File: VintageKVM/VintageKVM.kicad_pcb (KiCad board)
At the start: 2 copper layers, 164 parts, among them J1 Micro USB, J10 DE15_Receptacle_HighDensity_M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, J12 DE15_Receptacle_HighDensity_M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, J14 DE15_Receptacle_HighDensity_M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, J16 DE15_Receptacle_HighDensity_M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, J4 Conn_02x10_Odd_Even, J5 Conn_01x20_Pin, J6 Conn_01x20_Pin, J8 DE15_Receptacle_HighDensity_M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, Q1 BSS138, Q10 BSS138, Q2 BSS138, Q3 BSS138, Q4 BSS138, Q5 BSS138, Q6 BSS138, Q7 BSS138, Q8 BSS138, Q9 BSS138, U2 TS5V522CPWR, U3 TS5V522CPWR

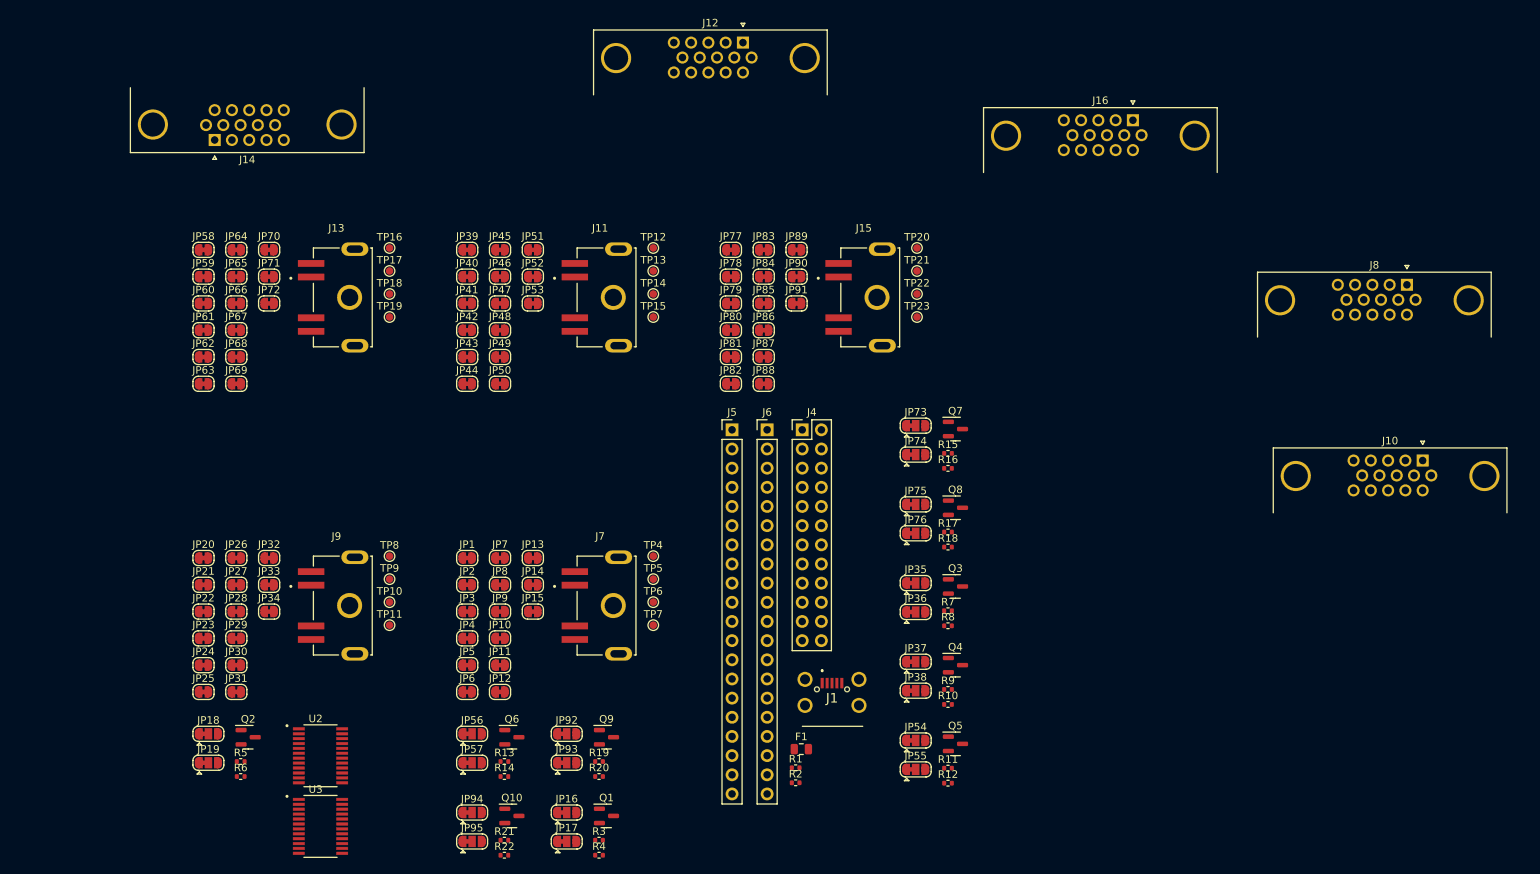
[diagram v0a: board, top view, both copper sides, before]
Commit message: started layout
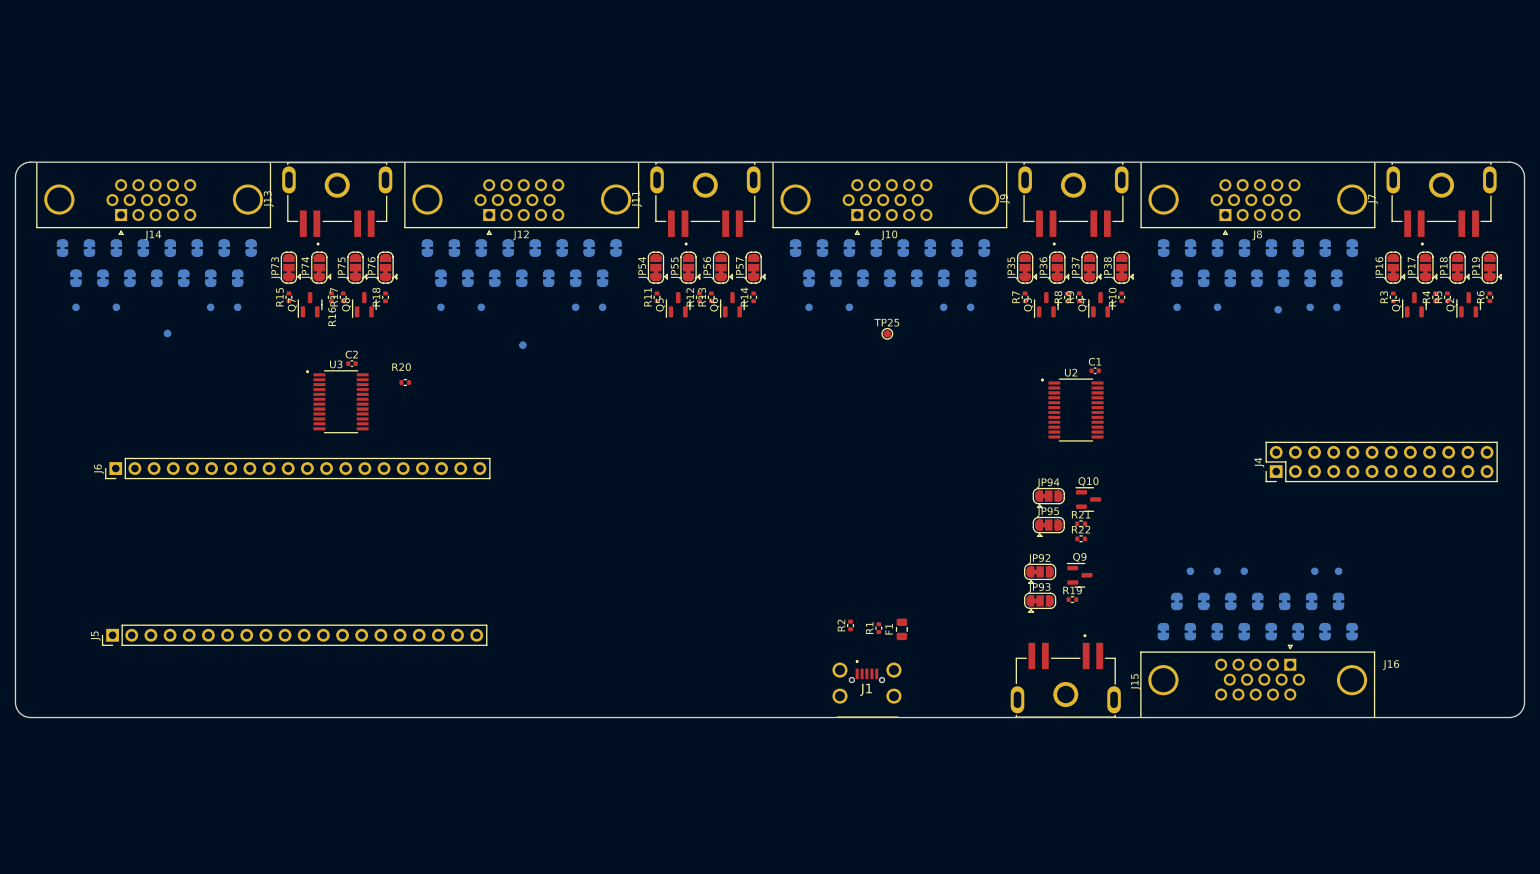
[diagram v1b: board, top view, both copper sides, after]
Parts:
- added C1: 100nF, Capacitor_SMD:C_0402_1005Metric, F.Cu at (183.1, 67.7)
- added C2: 100nF, Capacitor_SMD:C_0402_1005Metric, F.Cu at (84.6, 66.7)
- added TP24: TestPoint_Small, TestPoint:TestPoint_Pad_D1.0mm, B.Cu at (207.3, 59.5)
- added TP25: TestPoint_Small, TestPoint:TestPoint_Pad_D1.0mm, F.Cu at (155.6, 62.8)
- added TP26: TestPoint_Small, TestPoint:TestPoint_Pad_D1.0mm, B.Cu at (107.2, 64.2)
- added TP27: TestPoint_Small, TestPoint:TestPoint_Pad_D1.0mm, B.Cu at (60.1, 62.7)
- added TP28: TestPoint_Small, TestPoint:TestPoint_Pad_D1.0mm, B.Cu at (202.9, 94.2)
- JP1, JP10, JP11, JP12, JP13, JP14, JP15, JP2, JP20, JP21, JP22, JP23, JP24, JP25, JP26, JP27, JP28, JP29, JP3, JP30, JP31, JP32, JP33, JP34, JP39, JP4, JP40, JP41, JP42, JP43, JP44, JP45, JP46, JP47, JP48, JP49, JP5, JP50, JP51, JP52, JP53, JP58, JP59, JP6, JP60, JP61, JP62, JP63, JP64, JP65, JP66, JP67, JP68, JP69, JP7, JP70, JP71, JP72, JP77, JP78, JP79, JP8, JP80, JP81, JP82, JP83, JP84, JP85, JP86, JP87, JP88, JP89, JP9, JP90, JP91, TP10, TP11, TP12, TP13, TP14, TP15, TP16, TP17, TP18, TP19, TP20, TP21, TP22, TP23, TP4, TP5, TP6, TP7, TP8, TP9: moved to B.Cu
- moved JP19 182.1 mm to (235.4, 54.0), turned to 90 degrees
- moved R6 177.3 mm to (235.4, 57.9), turned to 90 degrees
- moved JP18 176.7 mm to (231.1, 54.0), turned to 90 degrees
- moved Q2 171.6 mm to (232.6, 58.9), turned to 90 degrees
- moved R5 171.4 mm to (229.8, 57.9), turned to 90 degrees
- moved JP17 136.9 mm to (226.9, 54.0), turned to 90 degrees
- moved R4 133.3 mm to (228.2, 57.9), turned to 90 degrees
- moved JP16 131.2 mm to (222.6, 54.0), turned to 90 degrees
- moved R3 127.5 mm to (222.6, 57.9), turned to 90 degrees
- moved Q1 126.7 mm to (225.4, 58.9), turned to 90 degrees
- moved JP1 124.3 mm to (217.2, 51.4), turned to 90 degrees
- moved JP3 123.5 mm to (213.6, 51.4), turned to 90 degrees
- moved J7 123.5 mm to (229.0, 44.0), turned to 90 degrees
- moved JP5 123.2 mm to (210.0, 51.4), turned to 90 degrees
- moved JP2 122.2 mm to (215.1, 55.4), turned to 90 degrees
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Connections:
- J4 pad 10: unconnected-(J4-Pin_10-Pad10) -> GND
- J4 pad 7: unconnected-(J4-Pin_7-Pad7) -> GND
- J4 pad 8: unconnected-(J4-Pin_8-Pad8) -> GND
- J6 pad 14: unconnected-(J6-Pin_14-Pad14) -> GPIO21
- J6 pad 4: unconnected-(J6-Pin_4-Pad4) -> 3v3_EN
- JP25 pad 1: GND -> Net-(JP25-A)
- JP44 pad 1: GND -> Net-(JP44-A)
- JP6 pad 1: GND -> Net-(JP6-A)
- JP63 pad 1: GND -> Net-(JP63-A)
- JP82 pad 1: GND -> Net-(JP82-A)
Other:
- board outline added: 200 x 73.6 mm
